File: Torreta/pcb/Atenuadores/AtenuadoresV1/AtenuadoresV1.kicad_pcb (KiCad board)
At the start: 4 copper layers, 86 x 66 mm, 15 parts, among them J1 Conn_Coaxial, J2 Conn_Coaxial, J3 Conn_Coaxial, J4 Conn_Coaxial, J5 Conn_Coaxial, J6 Conn_Coaxial

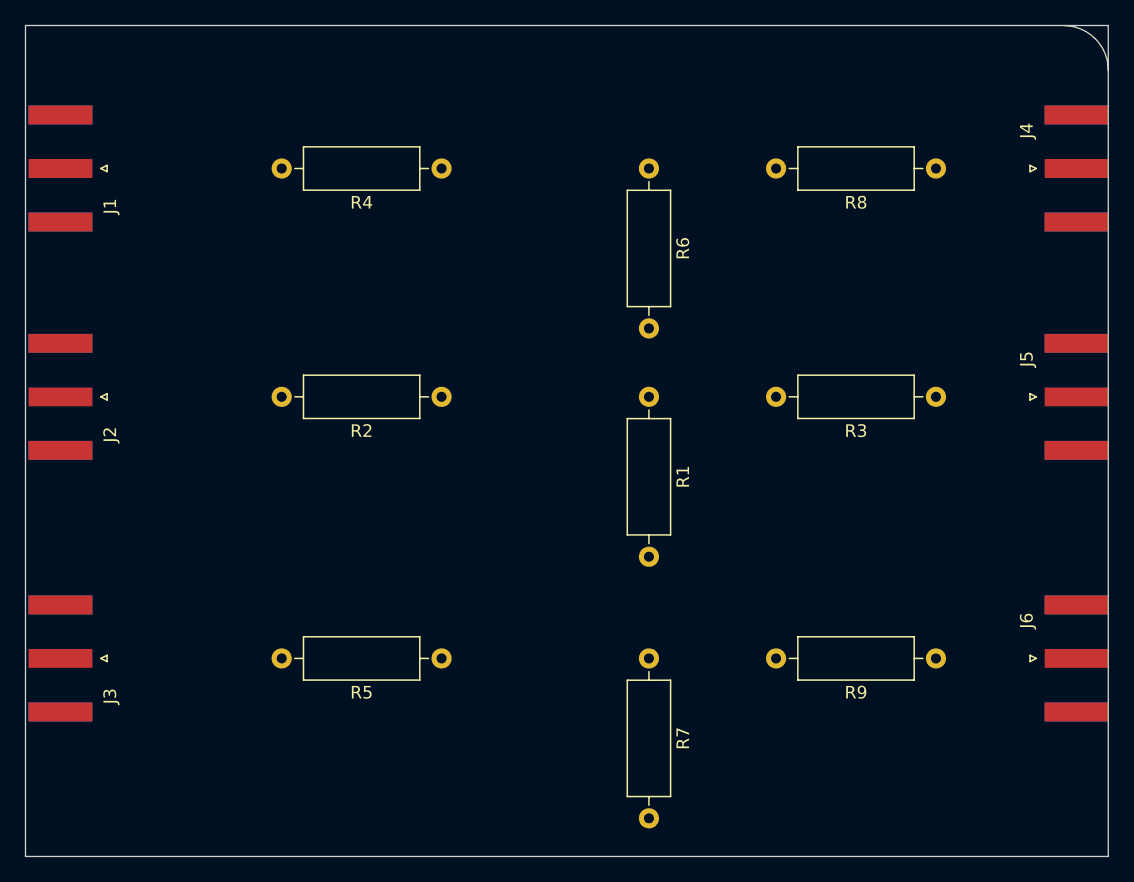
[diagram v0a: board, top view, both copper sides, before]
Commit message: preparación para optimización codigo
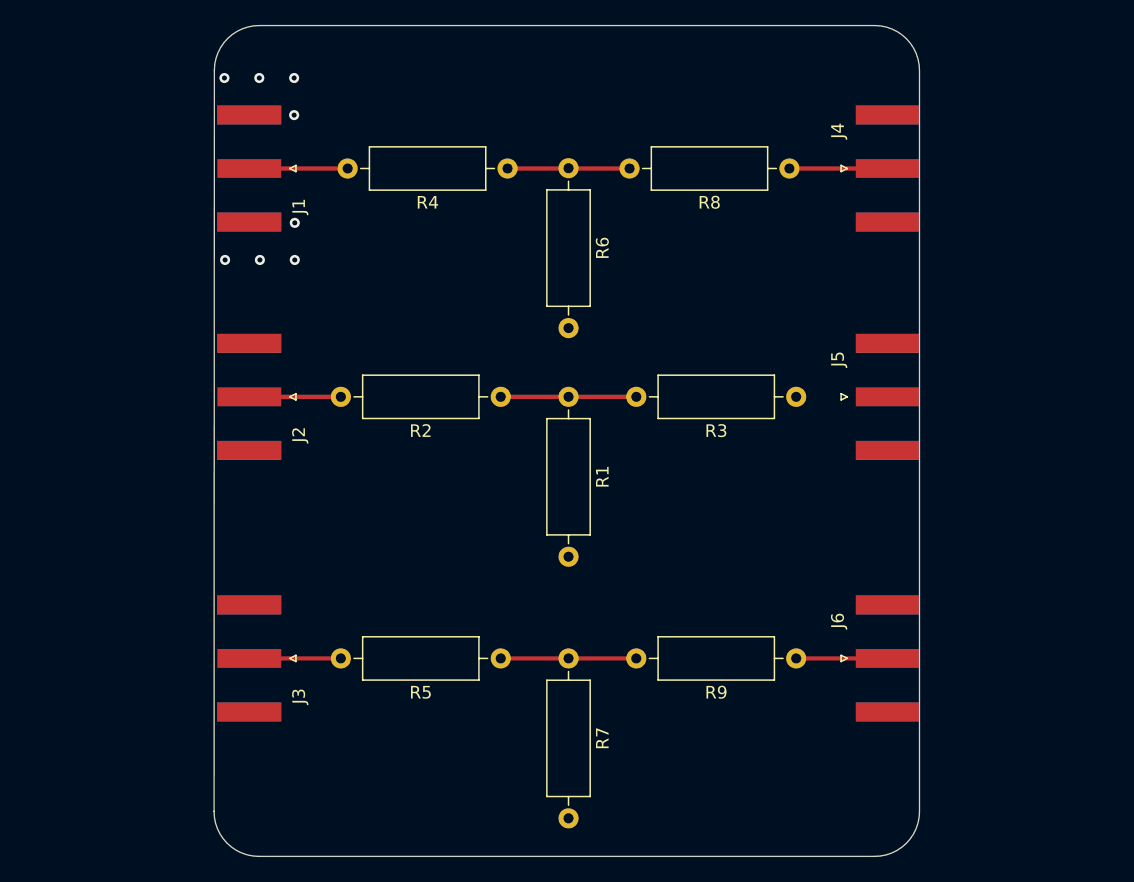
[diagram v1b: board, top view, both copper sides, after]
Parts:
- moved J1 15.0 mm to (187.8, 430.3)
- moved J2 15.0 mm to (187.8, 448.5)
- moved J3 15.0 mm to (187.8, 469.2)
- moved J4 15.0 mm to (238.5, 430.3)
- moved J5 15.0 mm to (238.5, 448.5)
- moved J6 15.0 mm to (238.5, 469.2)
- moved R8 11.6 mm to (230.7, 430.3)
- moved R3 11.1 mm to (231.2, 448.5)
- moved R9 11.1 mm to (231.2, 469.2)
- moved R6 6.39 mm to (213.1, 430.3)
- moved R1 6.39 mm to (213.1, 448.5)
- moved R7 6.39 mm to (213.1, 469.2)
- moved R4 5.24 mm to (208.3, 430.3)
- moved R2 4.70 mm to (207.7, 448.5)
- moved R5 4.70 mm to (207.7, 469.2)
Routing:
- net Net-(R5-Pad1): track 0.00 -> 10.8 mm
- net Net-(R1-Pad1): track 0.00 -> 10.8 mm
- net Net-(R4-Pad1): track 0.00 -> 9.71 mm
- net Salida1: track 0.00 -> 7.82 mm
- net Entrada1: track 0.00 -> 7.82 mm
- net Salida3: track 0.00 -> 7.28 mm
- net Entrada3: track 0.00 -> 7.28 mm
- net Entrada2: track 0.00 -> 7.28 mm
- net GND: vias 0 -> 3
- net (no net): vias 0 -> 5
- removed copper zone on In1.Cu, net GND
- removed copper zone on In2.Cu, net GND
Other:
- board size 86 x 66 mm -> 56 x 66 mm
